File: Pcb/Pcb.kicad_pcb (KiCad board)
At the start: 2 copper layers, 152.3 x 104.7 mm, 129 parts, among them J1 ISP, J2 TRRS, Q1 2N7002, SW1 SW_Push, SW10 SW_Push, SW11 SW_Push, SW12 SW_Push, SW13 SW_Push, SW14 SW_Push, SW15 SW_Push, SW16 SW_Push, SW17 SW_Push, SW18 SW_Push, SW19 SW_Push, SW2 SW2, SW20 SW_Push, SW21 SW_Push, SW22 SW_Push, SW23 SW_Push, SW24 SW_Push, SW25 SW_Push, SW26 SW_Push, SW27 SW_Push, SW28 SW_Push, SW29 SW_Push, SW3 SW_Push, SW4 SW_Push, SW5 SW_Push, SW6 SW_Push, SW7 SW_Push, SW8 SW_Push, SW9 SW_Push, U1 ProMicro

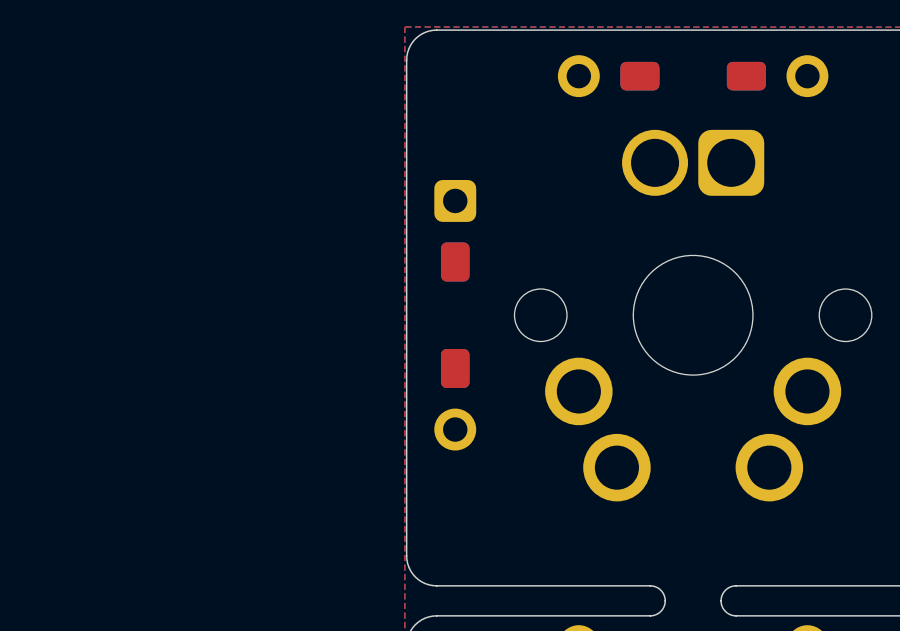
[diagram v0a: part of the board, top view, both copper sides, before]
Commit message: Moved diode
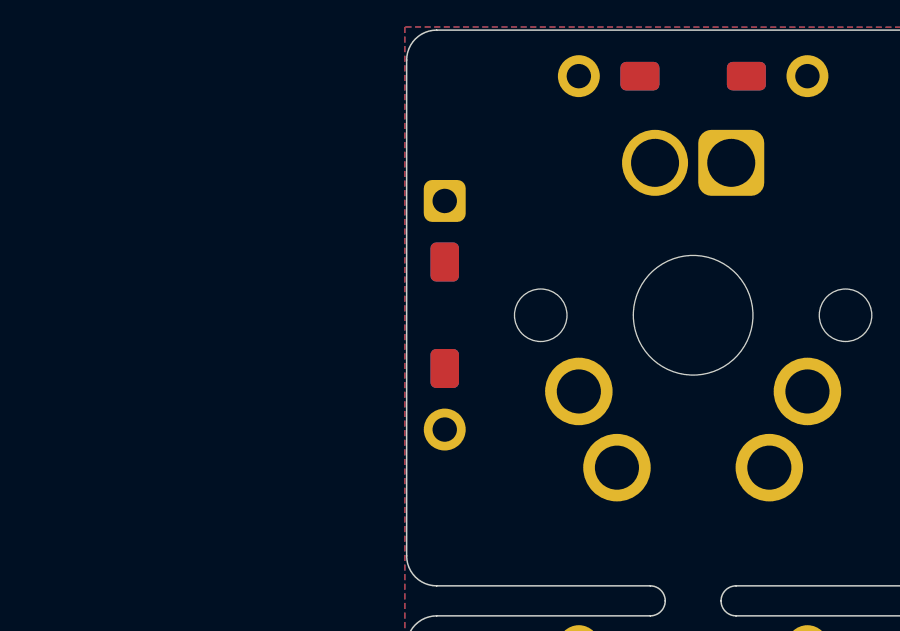
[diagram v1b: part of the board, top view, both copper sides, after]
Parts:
- moved D1 0.35 mm to (97.4, 53.9)
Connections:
- R29 pad 1: Net-(R29-Pad1) -> SDA
- R29 pad 2: SDA -> VCC
- R30 pad 1: Net-(R30-Pad1) -> VCC
- U1 pad 5: Net-(R29-Pad1) -> SDA
- U1 pad 6: Net-(R30-Pad1) -> SCL
